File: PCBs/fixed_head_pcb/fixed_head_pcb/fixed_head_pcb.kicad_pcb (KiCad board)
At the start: 2 copper layers, 50.2 x 47.1 mm, 2 parts, among them J1 DB15_Female_HighDensity, U1 Pick_and_place_pcb

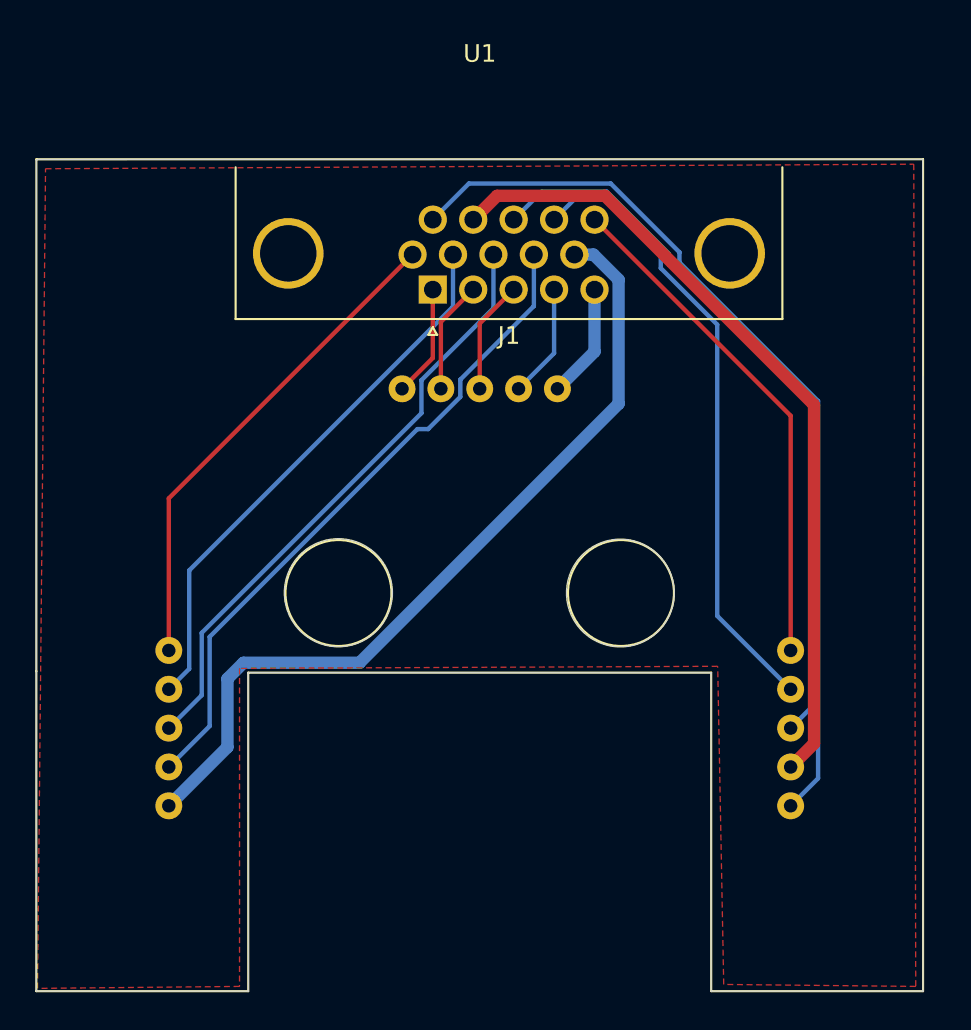
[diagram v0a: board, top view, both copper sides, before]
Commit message: modify kicad and freecad
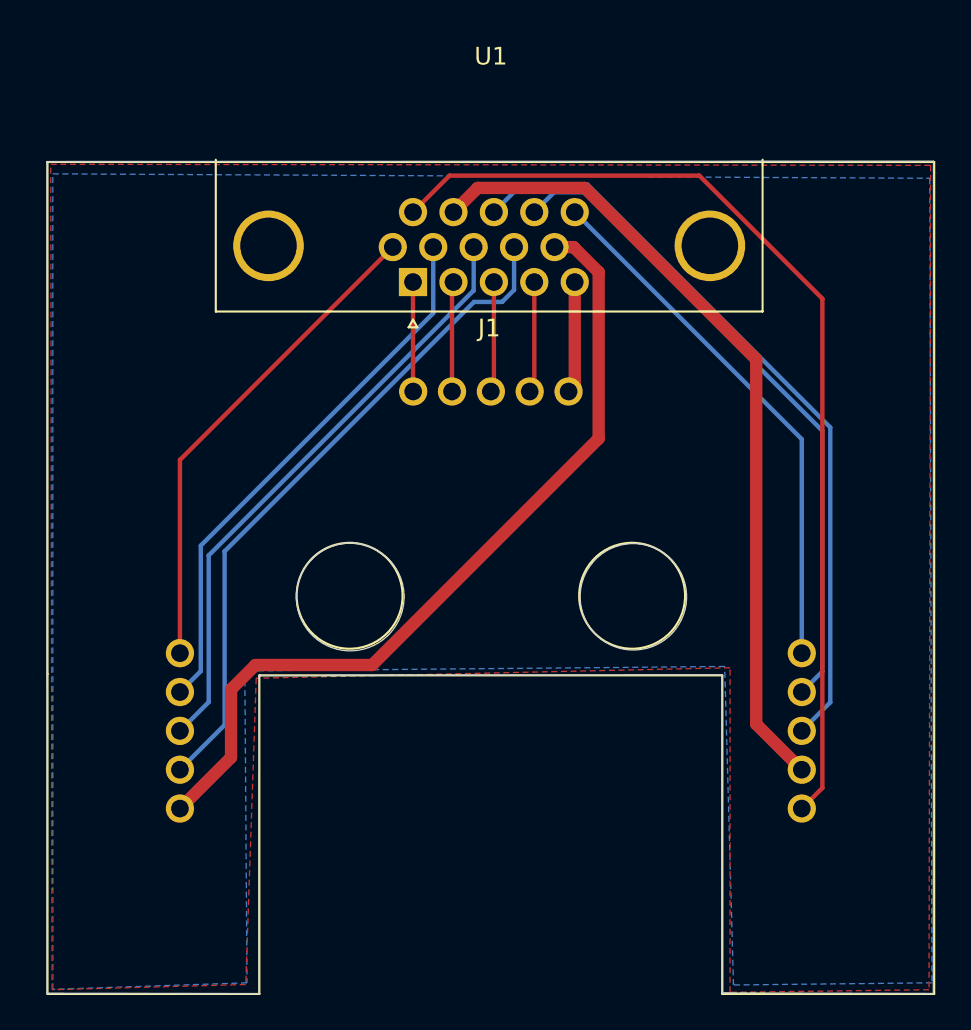
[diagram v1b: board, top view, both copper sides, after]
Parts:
- moved J1 1.20 mm to (143.4, 49.0)
- moved U1 0.65 mm to (147.8, 70.2)
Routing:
- net pwm: track 51.7 -> 56.3 mm
- net SCL: track 35.4 -> 37.7 mm
- net limZ: track 41.5 -> 43.3 mm
- net SDA: track 29.0 -> 30.3 mm
- added copper zone on B.Cu, net +3V3
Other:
- outline, holes or cut-outs redrawn
